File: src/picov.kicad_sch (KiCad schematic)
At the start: 50 parts, among them J1 USB_C_Receptacle_USB2.0_16P, J2 Conn_01x20, J3 Conn_01x20, J4 Conn_01x03, J5 Conn_01x06, SW1 SW_Push, SW2 SW_Push, U1 RP2040, U10 WS2812-2020, U11 WS2812-2020, U12 WS2812-2020, U13 WS2812-2020, U14 WS2812-2020, U15 WS2812-2020, U16 WS2812-2020, U17 WS2812-2020, U18 WS2812-2020, U19 WS2812-2020, U2 WS2812-2020, U3 W25Q16JVUXIQ_TR, U4 USBLC6-2SC6, U5 WS2812-2020, U6 WS2812-2020, U7 WS2812-2020, U8 WS2812-2020, U9 WS2812-2020, Y1 ABM8-272-T3

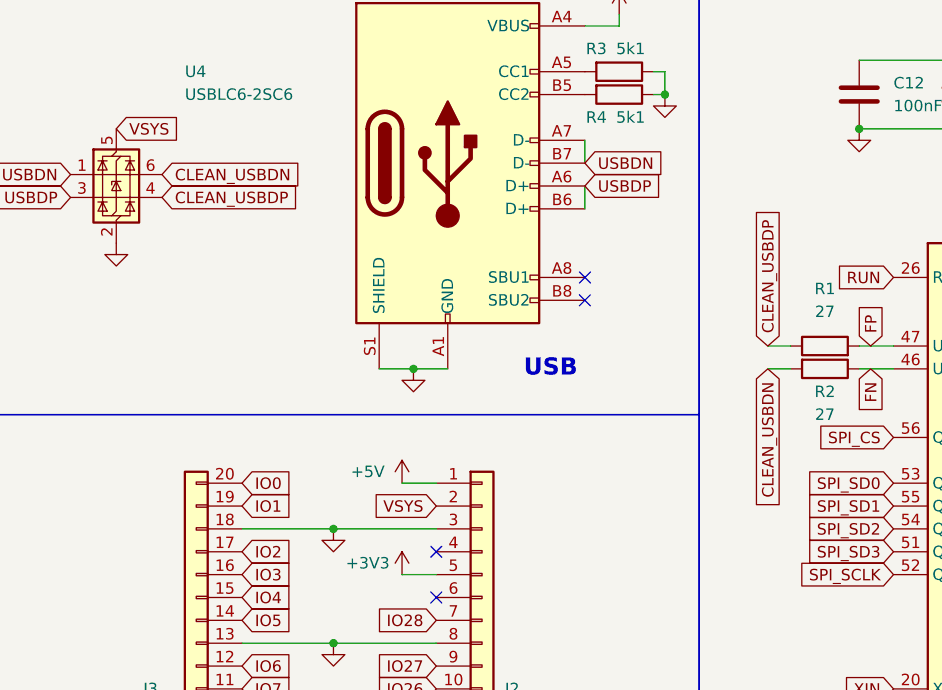
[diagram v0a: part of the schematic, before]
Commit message: changed some routing
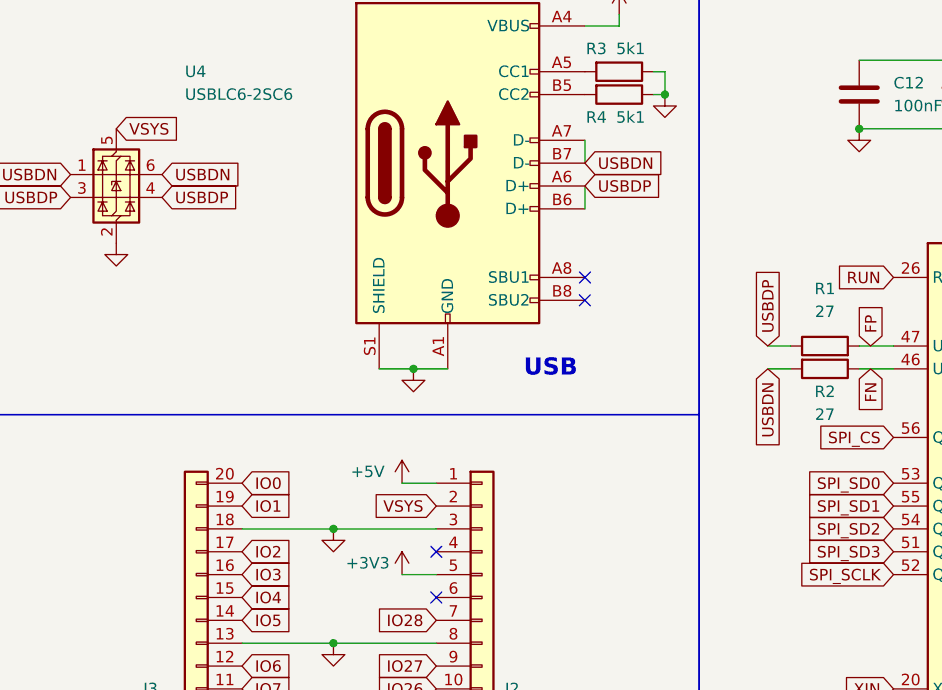
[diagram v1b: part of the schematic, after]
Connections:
- net CLEAN_USBDN is gone; now on net USBDN: R2.2, U4.6 (I/O1)
- net CLEAN_USBDP is gone; now on net USBDP: R1.1, U4.4 (I/O2)
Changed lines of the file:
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@@
 		)
 	)
-	(global_label "CLEAN_USBDP"
+	(global_label "USBDP"
 		(shape input)
 		(at 134.62 41.91 0)
@@
 		)
 		(property "Intersheetrefs" "${INTERSHEET_REFS}"
-			(at 150.789 41.91 0)
+			(at 143.9552 41.91 0)
 			(effects
 				(font
@@
 		)
 	)
-	(global_label "CLEAN_USBDP"
+	(global_label "USBDP"
 		(shape input)
 		(at 201.93 58.42 90)
@@
 		)
 		(property "Intersheetrefs" "${INTERSHEET_REFS}"
-			(at 201.93 42.251 90)
+			(at 201.93 49.0848 90)
 			(effects
 				(font
@@
 		)
 	)
-	(global_label "CLEAN_USBDN"
+	(global_label "USBDN"
 		(shape input)
 		(at 134.62 39.37 0)
@@
 		)
 		(property "Intersheetrefs" "${INTERSHEET_REFS}"
-			(at 150.8495 39.37 0)
+			(at 144.0157 39.37 0)
 			(effects
 				(font
@@
 		)
 	)
-	(global_label "CLEAN_USBDN"
+	(global_label "USBDN"
 		(shape input)
 		(at 201.93 60.96 270)
@@
 		)
 		(property "Intersheetrefs" "${INTERSHEET_REFS}"
-			(at 201.93 77.1895 90)
-			(effects
-				(font
+			(at 201.93 70.3557 90)
+			(effects
+				(font
